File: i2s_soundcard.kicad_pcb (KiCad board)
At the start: 4 copper layers, 83.1 x 50 mm, 21 parts, among them J1 Conn_01x08, J2 Conn_01x06, J3 Conn_01x05, J4 Conn_01x11, J5 Conn_01x04, U1 TLV320AIC3104IRHBT, U2 FSA2275UMX, U3 TPA2006D1DRBR, U4 FSA2275UMX, U5 TPA2006D1DRBR, U6 TLV7111830DSER, U7 TPD4E02B04DQAR, U8 TPD4E02B04DQAR

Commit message: Capitalize net names
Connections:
- net /LOL+ renamed /LOL_P
- net /LOL- renamed /LOL_N
- net /LOR+ renamed /LOR_P
- net /LOR- renamed /LOR_N
- net /bclk renamed /BCLK
- net /din renamed /DIN
- net /dout renamed /DOUT
- net /en1 renamed /EN1
- net /en2 renamed /EN2
- net /intmic+ renamed /INTMIC_P
- net /intmic- renamed /INTMIC_N
- net /iovdd renamed /IOVDD
- net /mclk renamed /MCLK
- net /mute renamed /MUTE
- net /reset renamed /RESET
- net /ring1 renamed /RING1
- net /ring2 renamed /RING2
- net /ring2_again renamed /RING2_AGAIN
- net /sca renamed /SCA
- net /scl renamed /SCL
- net /sel renamed /SEL
- net /sleeve renamed /SLEEVE
- net /tip renamed /TIP
- net /v1.8 renamed /VCC1.8
- net /v3.3 renamed /VCC3.3
- net /vbat renamed /VBAT_3.7
- net /wclk renamed /WCLK
- net /~shutdown renamed /~SHUTDOWN
- net Net-(J1-Pad7) renamed /DETECT?

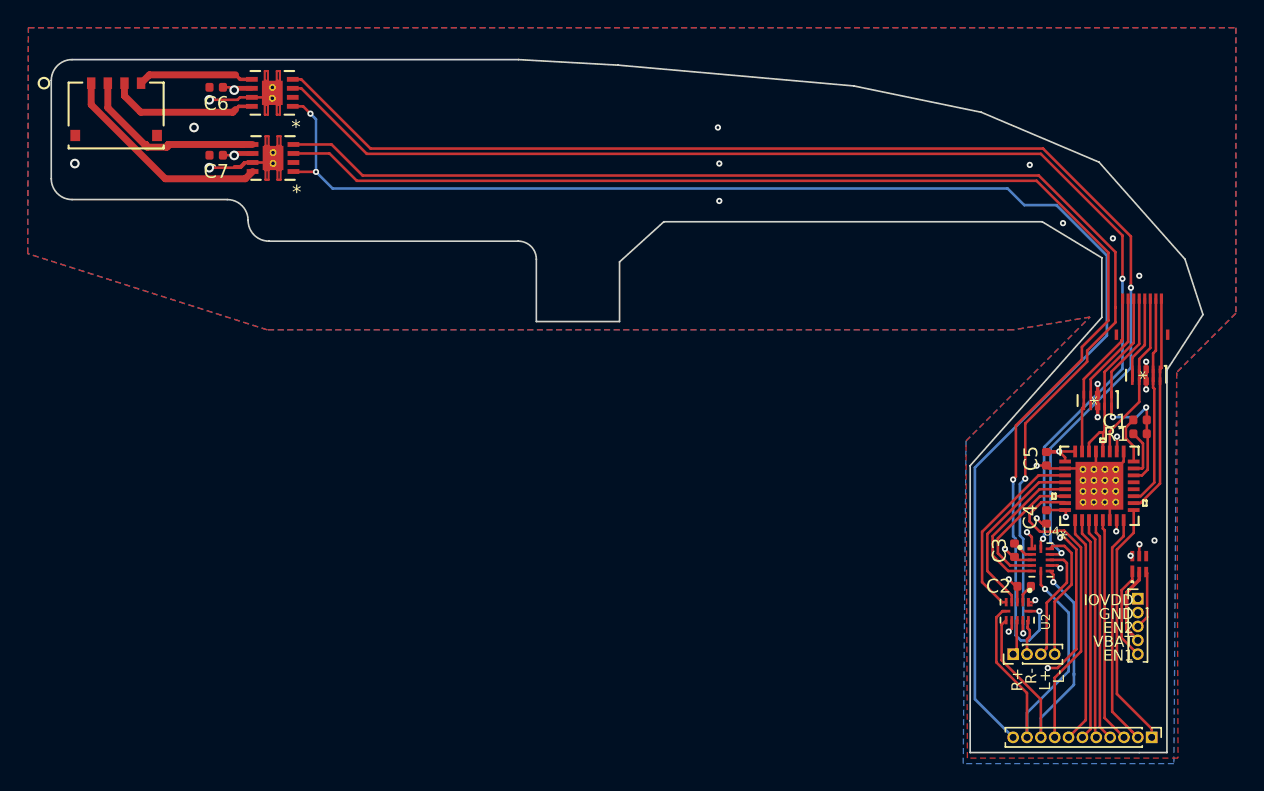
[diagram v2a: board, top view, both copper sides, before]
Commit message: Lots of schematic cleanup and board tweaking
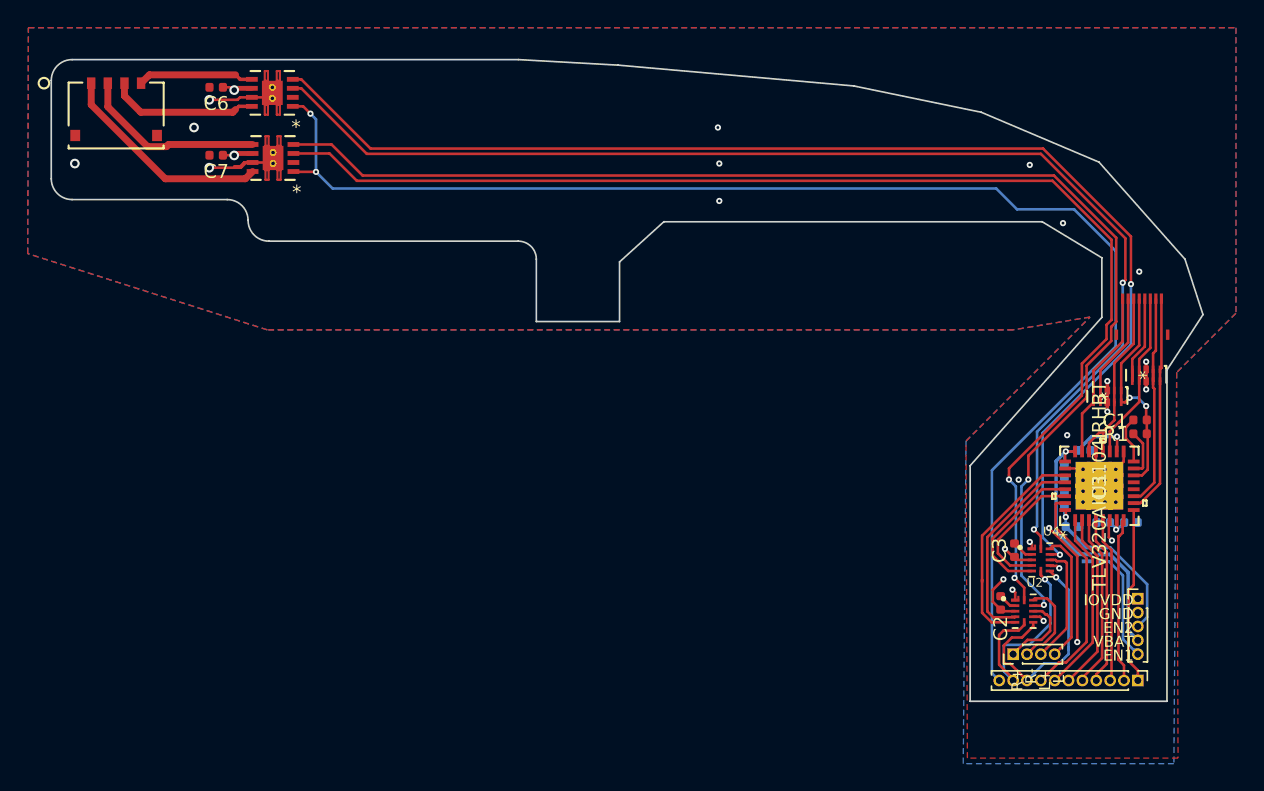
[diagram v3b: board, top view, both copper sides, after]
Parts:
- added C10: 10uF, Capacitor_SMD:C_0402_1005Metric, B.Cu at (163.7, 91.7)
- added C11: 100nF, Capacitor_SMD:C_0402_1005Metric, B.Cu at (165.7, 91.7)
- added C8: 0.1uF, Capacitor_SMD:C_0402_1005Metric, B.Cu at (161.5, 92.0)
- added C9: 220nF, Capacitor_SMD:C_0402_1005Metric, B.Cu at (162.3, 86.5)
- C4: value 1uF -> 10uF; moved to B.Cu
- C5: value 1uF -> 22uF; moved to B.Cu
- U6: moved to B.Cu
- moved J4 4.22 mm to (166.2, 103.1)
- moved U6 3.28 mm to (163.1, 94.0), turned to 180 degrees
- moved C2 2.08 mm to (156.3, 97.5), turned to 270 degrees
- moved C4 1.84 mm to (160.9, 90.0), turned to 270 degrees
- moved C5 1.58 mm to (160.9, 88.0)
- moved U8 0.76 mm to (164.0, 82.6)
- moved U2 0.50 mm to (158.0, 98.1), turned to 0 degrees
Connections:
- net /VCC3.3 renamed /VCC3.0
- J3 pad 3: /EN2 -> /EN1
- J3 pad 5: /EN1 -> /EN2
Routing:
- net /SEL: track 24.5 -> 16.9 mm
- net /MUTE: track 23.6 -> 17.0 mm
- net /RESET: track 22.5 -> 16.0 mm
- net /VBAT_3.7: track 27.5 -> 33.1 mm
- net /spkr_amp_left/SLO+: track 96.6 -> 91.2 mm
- net /SCA: track 17.9 -> 12.7 mm
- net /SCL: track 16.8 -> 12.0 mm
- net /~SHUTDOWN: track 106.9 -> 102.5 mm
- net /DOUT: track 16.3 -> 11.9 mm
- net GND: track 47.8 -> 43.8 mm, vias 24 -> 23
- net /EN2: track 4.26 -> 8.18 mm
- net /DIN: track 16.1 -> 12.2 mm
- net /LOR_N: track 2.64 -> 6.43 mm
- net /VCC1.8: track 7.85 -> 4.22 mm, vias 2 -> 1
- net /WCLK: track 15.9 -> 12.6 mm
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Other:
- board size 83.1 x 50 mm -> 83.1 x 46.3 mm
